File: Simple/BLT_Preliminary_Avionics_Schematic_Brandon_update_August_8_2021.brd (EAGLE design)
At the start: 118.1 x 61 mm, 12 parts

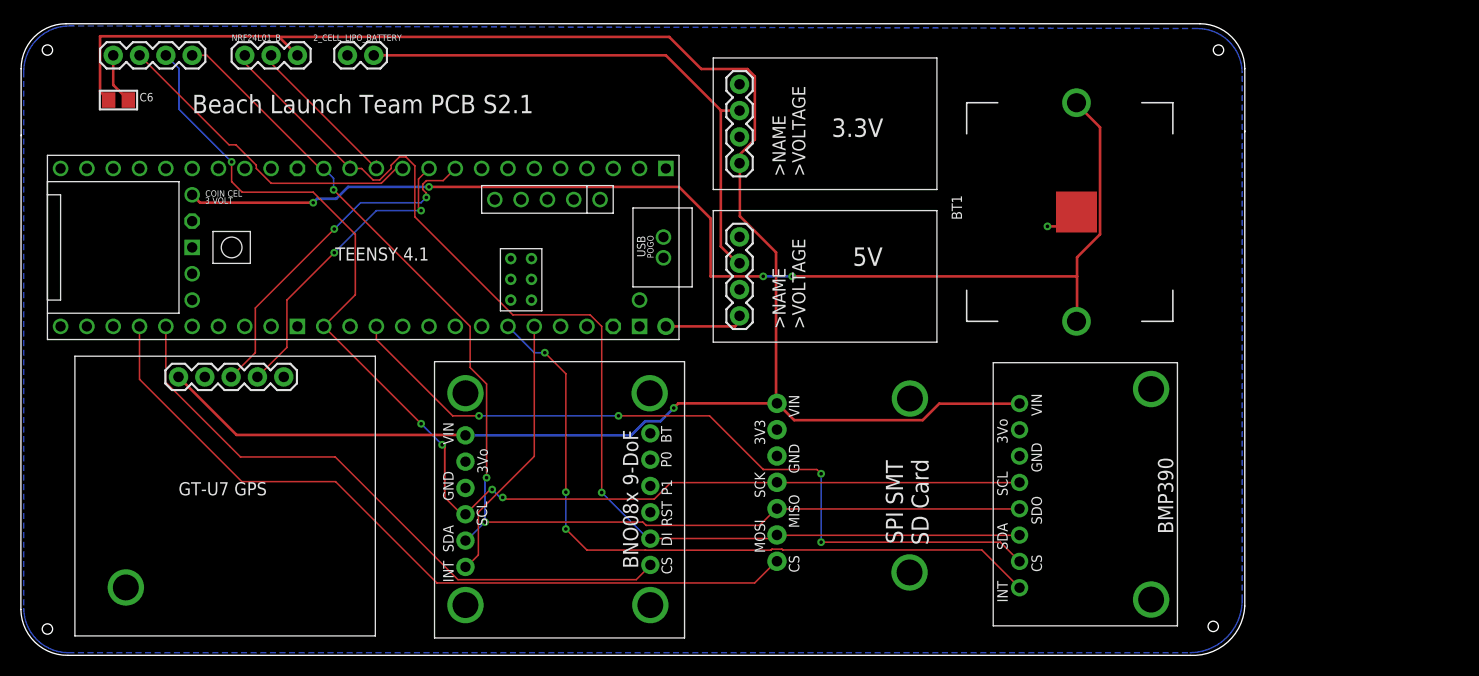
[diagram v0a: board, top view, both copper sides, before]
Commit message: Updated files
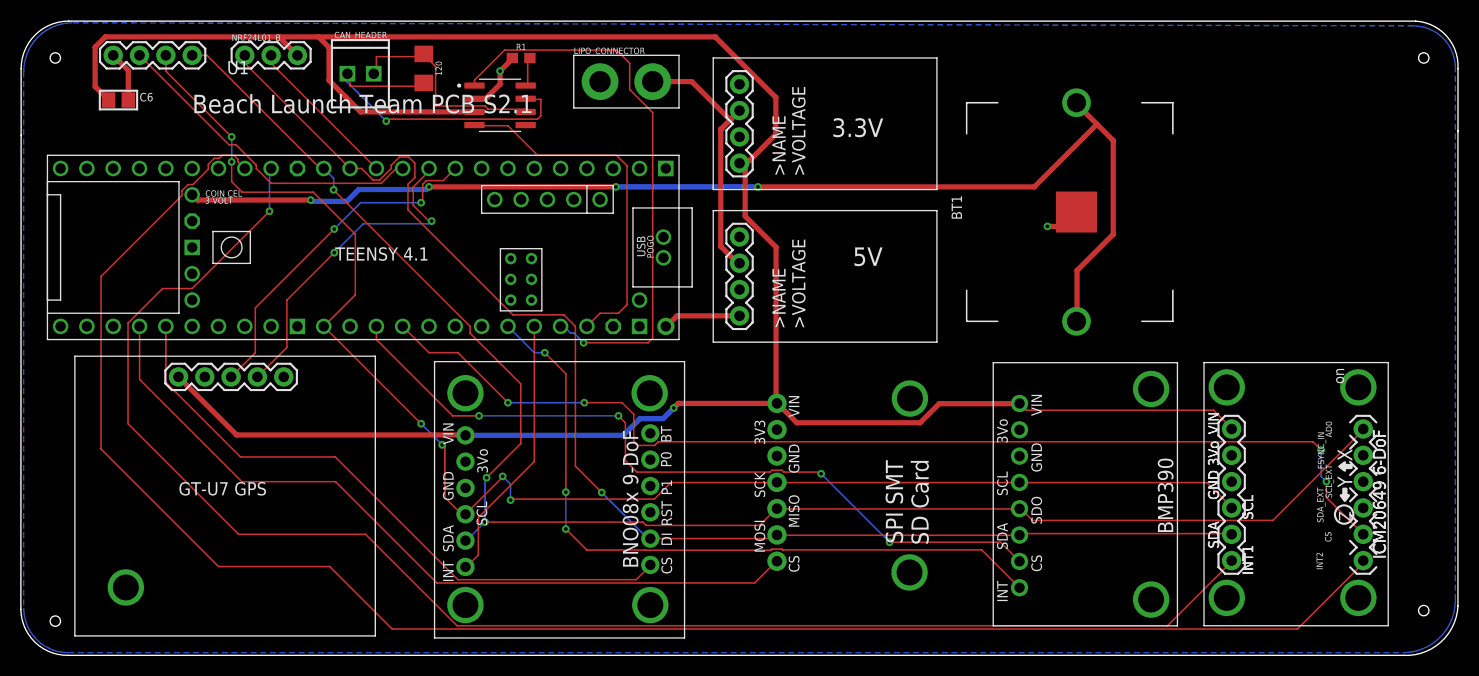
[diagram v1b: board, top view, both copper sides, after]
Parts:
- removed 2_CELL_LIPO_BATTERY: (no value), SparkFun-Connectors:1X02
- added 120: (no value), SparkFun-Resistors:1206
- added CAN_HEADER: (no value), SparkFun-Connectors:1X02_2.54_SCREWTERM
- added LIPO_CONNECTOR: (no value), SparkFun-Connectors:1X02_XTRA_BIG
- added R1: 10k, SparkFun-Resistors:0603
- added U$8: ICM20XXX, BLTFootprints:1X06
- added U1: SN65HVD230, SN65HVD230:SOIC127P599X175-8N
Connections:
- new net CANH: 120.2, CAN_HEADER.P2, U1.7
- new net CANL: 120.1, CAN_HEADER.P1, U1.6
- new net CANRX: U$1.23-A9/CRX1/MCLK1, U1.4
- new net CANTX: U$1.22-A8/CTX1, U1.1
- new net CS3: U$1.16-A2/RX4/SCL1, U$8.CS
- new net ICMINT1: U$1.24-A10/TX6/SCL2, U$8.INT1
- new net ICMINT2: U$1.25-A11/RX6/SDA2, U$8.INT2
- new net SN65RS: R1.2, U1.8
- net 3.3V: now also U$8.VIN, U1.3
- net BAT+: now also LIPO_CONNECTOR.2; no longer 2_CELL_LIPO_BATTERY.2
- net GND: now also LIPO_CONNECTOR.1, R1.1, U$8.GND, U1.2; no longer 2_CELL_LIPO_BATTERY.1
- net MISO: now also U$8.AD0
- net MOSI: now also U$8.SDA
- net SCK: now also U$8.SCL
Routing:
- net ICMINT2: track 0.00 -> 168.5 mm
- net ICMINT1: track 0.00 -> 149.3 mm, vias 0 -> 1
- net CS3: track 0.00 -> 105.2 mm, vias 0 -> 4
- net CANTX: track 0.00 -> 54.4 mm, vias 0 -> 1
- net 3.3V: track 193.7 -> 237.4 mm
- net MISO: track 113.0 -> 153.0 mm
- net CANRX: track 0.00 -> 34.5 mm
- net CANH: track 0.00 -> 33.0 mm, vias 0 -> 1
- net BAT+: track 53.2 -> 25.5 mm
- net SCK: track 118.6 -> 142.2 mm, vias 5 -> 6
- net CANL: track 0.00 -> 21.0 mm
- net MOSI: track 109.9 -> 129.0 mm
- net GND: track 8.30 -> 14.6 mm, vias 1 -> 2
- net SN65RS: track 0.00 -> 2.83 mm
- net TX2: track 30.6 -> 32.3 mm
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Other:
- board size 118.1 x 61 mm -> 138.7 x 61.2 mm
